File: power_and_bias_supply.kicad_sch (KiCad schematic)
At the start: 42 parts, among them Q501 2N7002, U501 MCP6L02x-xSN, U502 LM2733YMFX/NOPB, U503 TPS22944DCKR, X5 Conn_Coaxial

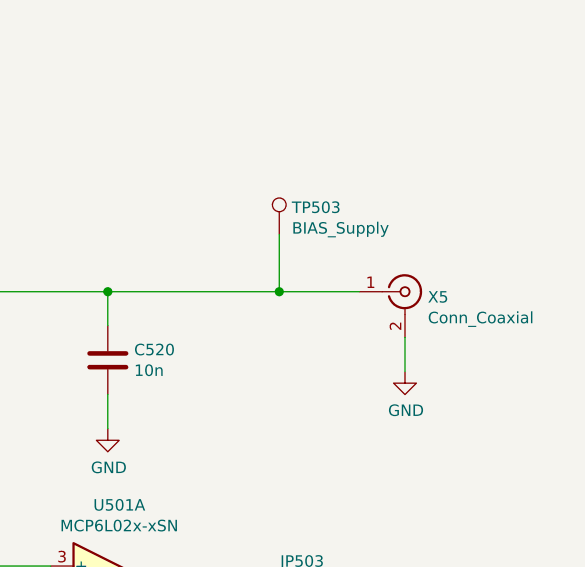
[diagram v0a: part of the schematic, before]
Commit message: worked on bom. some changes. added license
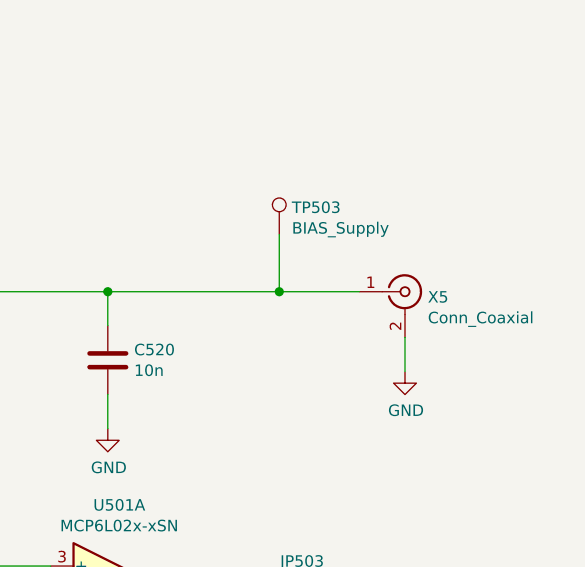
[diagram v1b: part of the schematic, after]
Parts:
- C501, C503, C504, C505, C520, C550, C553, C554, C560, C568, C569, Q501, R500, R501, R502, R503, R504, R505, R506, R507, R508, R509, R512, R516: JLC_placed_by (none) -> yes
- D500, L500, L501, U501, U503, X5: JLC_placed_by (none) -> no
- JP500, JP501, JP502, JP503, JP504, JP505, JP506, TP502, TP503, TP504, TP505: JLC_placed_by (none) -> never
- U502: JLC_placed_by (none) -> yes; JLCplace (none) -> C527399
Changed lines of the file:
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@@
+      (effects (font (size 1.27 1.27)) hide)
+    )
+    (property "JLC_placed_by" "never" (id 5) (at 120.65 38.1 0)
       (effects (font (size 1.27 1.27)) hide)
     )
@@
       (effects (font (size 1.27 1.27)) hide)
     )
+    (property "JLC_placed_by" "no" (id 9) (at 254 54.61 0)
+      (effects (font (size 1.27 1.27)) hide)
+    )
     (pin "1")
     (pin "2")
@@
       (effects (font (size 1.27 1.27)) hide)
     )
+    (property "JLC_placed_by" "yes" (id 10) (at 207.01 127 0)
+      (effects (font (size 1.27 1.27)) hide)
+    )
     (pin "1")
     (pin "2")
@@
     )
     (property "JLCType" "MCP6L02T-E/SN" (id 8) (at 177.8 144.78 0)
+      (effects (font (size 1.27 1.27)) hide)
+    )
+    (property "JLC_placed_by" "no" (id 9) (at 177.8 144.78 0)
       (effects (font (size 1.27 1.27)) hide)
     )
@@
     )
     (property "Supplier" "Mouser" (id 5) (at 46.99 72.39 0)
+      (effects (font (size 1.27 1.27)) hide)
+    )
+    (property "JLC_placed_by" "no" (id 6) (at 46.99 72.39 0)
       (effects (font (size 1.27 1.27)) hide)
     )
@@
       (effects (font (size 1.27 1.27)) hide)
     )
+    (property "JLC_placed_by" "never" (id 5) (at 64.77 41.91 0)
+      (effects (font (size 1.27 1.27)) hide)
+    )
     (pin "1")
     (pin "2")
@@
     )
     (property "JLCplace" "C17673" (id 9) (at 119.38 87.63 0)
+      (effects (font (size 1.27 1.27)) hide)
+    )
+    (property "JLC_placed_by" "yes" (id 10) (at 119.38 87.63 0)
       (effects (font (size 1.27 1.27)) hide)
     )
@@
       (effects (font (size 1.27 1.27)) hide)
     )
+    (property "JLC_placed_by" "no" (id 9) (at 222.25 87.63 0)
+      (effects (font (size 1.27 1.27)) hide)
+    )
     (pin "1")
     (pin "2")
@@
     )
     (property "JLCplace" "C26108" (id 9) (at 189.23 80.01 0)
+      (effects (font (size 1.27 1.27)) hide)
+    )
+    (property "JLC_placed_by" "yes" (id 10) (at 189.23 80.01 0)
       (effects (font (size 1.27 1.27)) hide)
     )
@@
       (effects (font (size 1.27 1.27)) hide)
     )
+    (property "JLC_placed_by" "yes" (id 10) (at 143.51 72.39 0)
+      (effects (font (size 1.27 1.27)) hide)
+    )
     (pin "1")
     (pin "2")
@@
     )
     (property "JLCplace" "C29823" (id 9) (at 104.14 147.32 0)
+      (effects (font (size 1.27 1.27)) hide)
+    )
+    (property "JLC_placed_by" "yes" (id 10) (at 104.14 147.32 0)
       (effects (font (size 1.27 1.27)) hide)
     )
@@
       (effects (font (size 1.27 1.27)) hide)
     )
+    (property "JLC_placed_by" "never" (id 5) (at 242.57 87.63 0)
+      (effects (font (size 1.27 1.27)) hide)
+    )
     (pin "1")
     (pin "2")
@@
     )
     (property "JLCplace" "C17514" (id 9) (at 189.23 95.25 0)
+      (effects (font (size 1.27 1.27)) hide)
+    )
+    (property "JLC_placed_by" "yes" (id 10) (at 189.23 95.25 0)
       (effects (font (size 1.27 1.27)) hide)
     )
@@
       (effects (font (size 1.27 1.27)) hide)
     )
+    (property "JLC_placed_by" "yes" (id 10) (at 173.99 80.01 0)
+      (effects (font (size 1.27 1.27)) hide)
+    )
     (pin "1")
     (pin "2")
@@
     )
     (property "JLCplace" "C46653" (id 9) (at 207.01 88.9 0)
+      (effects (font (size 1.27 1.27)) hide)
+    )
+    (property "JLC_placed_by" "yes" (id 10) (at 207.01 88.9 0)
       (effects (font (size 1.27 1.27)) hide)
     )
@@
       (effects (font (size 1.27 1.27)) hide)
     )
+    (property "JLC_placed_by" "no" (id 9) (at 78.74 41.91 0)
+      (effects (font (size 1.27 1.27)) hide)
+    )
     (pin "1")
     (pin "2")
@@
       (effects (font (size 1.27 1.27)) hide)
     )
+    (property "JLC_placed_by" "yes" (id 10) (at 90.17 95.25 0)
+      (effects (font (size 1.27 1.27)) hide)
+    )
     (pin "1")
     (pin "2")
@@
       (effects (font (size 1.27 1.27)) hide)
     )
+    (property "JLC_placed_by" "never" (id 5) (at 240.03 48.26 0)
+      (effects (font (size 1.27 1.27)) hide)
+    )
     (pin "1")
   )
@@
       (effects (font (size 1.27 1.27)) hide)
     )
+    (property "JLC_placed_by" "yes" (id 10) (at 147.32 85.09 0)
+      (effects (font (size 1.27 1.27)) hide)
+    )
     (pin "1")
     (pin "2")
@@
     )
     (property "JLCplace" "C28323" (id 9) (at 93.98 147.32 0)
+      (effects (font (size 1.27 1.27)) hide)
+    )
+    (property "JLC_placed_by" "yes" (id 10) (at 93.98 147.32 0)
       (effects (font (size 1.27 1.27)) hide)
     )
@@
       (effects (font (size 1.27 1.27)) hide)
     )
+    (property "JLC_placed_by" "no" (id 9) (at 222.25 125.73 0)
+      (effects (font (size 1.27 1.27)) hide)
+    )
     (pin "5")
     (pin "6")
@@
       (effects (font (size 1.27 1.27)) hide)
     )
+    (property "JLC_placed_by" "yes" (id 10) (at 21.59 91.44 0)
+      (effects (font (size 1.27 1.27)) hide)
+    )
     (pin "1")
     (pin "2")
@@
       (effects (font (size 1.27 1.27)) hide)
     )
+    (property "JLC_placed_by" "yes" (id 10) (at 173.99 95.25 0)
+      (effects (font (size 1.27 1.27)) hide)
+    )
     (pin "1")
     (pin "2")
@@
     )
     (property "JLCplace" "C29823" (id 9) (at 48.26 161.29 0)
+      (effects (font (size 1.27 1.27)) hide)
+    )
+    (property "JLC_placed_by" "yes" (id 10) (at 48.26 161.29 0)
       (effects (font (size 1.27 1.27)) hide)
     )
@@
       (effects (font (size 1.27 1.27)) hide)
     )
+    (property "JLC_placed_by" "no" (id 9) (at 71.12 72.39 0)
+      (effects (font (size 1.27 1.27)) hide)
+    )
     (pin "1")
     (pin "2")
@@
       (effects (font (size 1.27 1.27)) hide)
     )
+    (property "JLC_placed_by" "yes" (id 10) (at 152.4 91.44 0)
+      (effects (font (size 1.27 1.27)) hide)
+    )
     (pin "1")
     (pin "2")
@@
     )
     (property "JLCplace" "C1716" (id 9) (at 78.74 80.01 0)
+      (effects (font (size 1.27 1.27)) hide)
+    )
+    (property "JLC_placed_by" "yes" (id 10) (at 78.74 80.01 0)
       (effects (font (size 1.27 1.27)) hide)
     )
@@
       (effects (font (size 1.27 1.27)) hide)
     )
+    (property "JLC_placed_by" "no" (id 6) (at 129.54 72.39 0)
+      (effects (font (size 1.27 1.27)) hide)
+    )
     (pin "1")
     (pin "2")
@@
       (effects (font (size 1.27 1.27)) hide)
     )
+    (property "JLC_placed_by" "yes" (id 10) (at 78.74 95.25 0)
+      (effects (font (size 1.27 1.27)) hide)
+    )
     (pin "1")
     (pin "2")
@@
     )
     (property "JLCplace" "C29823" (id 9) (at 101.6 87.63 0)
+      (effects (font (size 1.27 1.27)) hide)
+    )
+    (property "JLC_placed_by" "yes" (id 10) (at 101.6 87.63 0)
       (effects (font (size 1.27 1.27)) hide)
     )
@@
       (effects (font (size 1.27 1.27)) hide)
     )
+    (property "JLC_placed_by" "yes" (id 10) (at 181.61 72.39 0)
+      (effects (font (size 1.27 1.27)) hide)
+    )
     (pin "1")
     (pin "2")
@@
       (effects (font (size 1.27 1.27)) hide)
     )
+    (property "JLC_placed_by" "never" (id 5) (at 58.42 148.59 0)
+      (effects (font (size 1.27 1.27)) hide)
+    )
     (pin "1")
   )
@@
     )
     (property "Supplier" "--" (id 4) (at 93.98 134.62 0)
+      (effects (font (size 1.27 1.27)) hide)
+    )
+    (property "JLC_placed_by" "never" (id 5) (at 93.98 134.62 0)
       (effects (font (size 1.27 1.27)) hide)
     )
@@
       (effects (font (size 1.27 1.27)) hide)
     )
+    (property "JLC_placed_by" "yes" (id 9) (at 46.99 85.09 0)
+      (effects (font (size 1.27 1.27)) hide)
+    )
+    (property "JLCplace" "C527399" (id 10) (at 46.99 85.09 0)
+      (effects (font (size 1.27 1.27)) hide)
+    )
     (pin "1")
     (pin "2")
@@
     )
     (property "JLCplace" "C49678" (id 9) (at 40.64 46.99 0)
+      (effects (font (size 1.27 1.27)) hide)
+    )
+    (property "JLC_placed_by" "yes" (id 10) (at 40.64 46.99 0)
       (effects (font (size 1.27 1.27)) hide)
     )
@@
       (effects (font (size 1.27 1.27)) hide)
     )
+    (property "JLC_placed_by" "never" (id 5) (at 90.17 104.14 0)
+      (effects (font (size 1.27 1.27)) hide)
+    )
     (pin "1")
     (pin "2")
@@
       (effects (font (size 1.27 1.27)) hide)
     )
+    (property "JLC_placed_by" "never" (id 5) (at 134.62 19.05 0)
+      (effects (font (size 1.27 1.27)) hide)
+    )
     (pin "1")
     (pin "2")
@@
     )
     (property "JLCplace" "C17414" (id 9) (at 110.49 36.83 0)
+      (effects (font (size 1.27 1.27)) hide)
+    )
+    (property "JLC_placed_by" "yes" (id 10) (at 110.49 36.83 0)
       (effects (font (size 1.27 1.27)) hide)
     )
@@
       (effects (font (size 1.27 1.27)) hide)
     )
+    (property "JLC_placed_by" "never" (id 5) (at 127 41.91 0)
+      (effects (font (size 1.27 1.27)) hide)
+    )
     (pin "1")
     (pin "2")
@@
       (effects (font (size 1.27 1.27)) hide)
     )
+    (property "JLC_placed_by" "never" (id 5) (at 147.32 99.06 0)
+      (effects (font (size 1.27 1.27)) hide)
+    )
     (pin "1")
     (pin "2")
@@
       (effects (font (size 1.27 1.27)) hide)
     )
+    (property "JLC_placed_by" "yes" (id 10) (at 167.64 144.78 0)
+      (effects (font (size 1.27 1.27)) hide)
+    )
     (pin "1")
     (pin "2")
@@
     )
     (property "JLCplace" "C17556" (id 9) (at 90.17 80.01 0)
+      (effects (font (size 1.27 1.27)) hide)
+    )
+    (property "JLC_placed_by" "yes" (id 10) (at 90.17 80.01 0)
       (effects (font (size 1.27 1.27)) hide)
     )
@@
     )
     (property "JLCplace" "C1710" (id 9) (at 220.98 62.23 0)
+      (effects (font (size 1.27 1.27)) hide)
+    )
+    (property "JLC_placed_by" "yes" (id 10) (at 220.98 62.23 0)
       (effects (font (size 1.27 1.27)) hide)
     )
@@
       (effects (font (size 1.27 1.27)) hide)
     )
+    (property "JLC_placed_by" "never" (id 5) (at 242.57 125.73 0)
+      (effects (font (size 1.27 1.27)) hide)
+    )
